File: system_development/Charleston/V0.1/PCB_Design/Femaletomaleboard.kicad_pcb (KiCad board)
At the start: 2 copper layers, 64.4 x 118.3 mm, 7 parts, among them SW2 MC74VHC1G66DFT1G

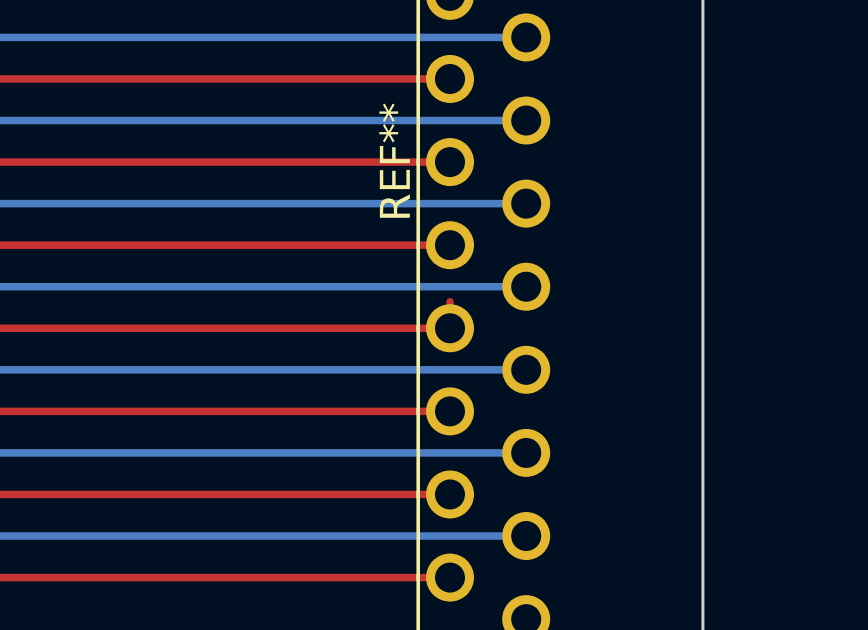
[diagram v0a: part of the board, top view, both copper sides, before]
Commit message: femaletomaleboard
Fingers crossed final version
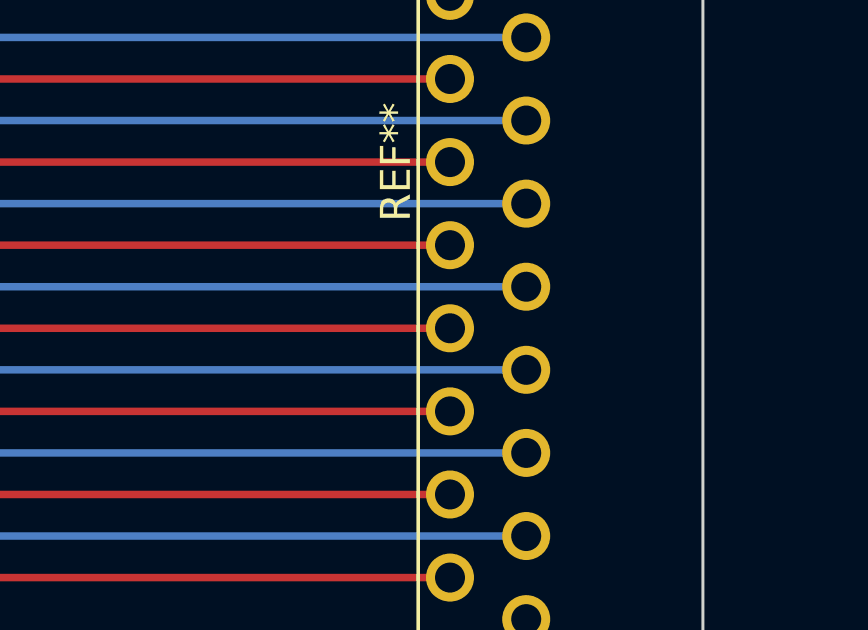
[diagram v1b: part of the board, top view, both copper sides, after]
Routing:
- net (no net): track 2812.3 -> 2811.5 mm
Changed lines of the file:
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@@
   (segment (start 142.325948 110.855) (end 142.235473 110.764525) (width 0.25) (layer "F.Cu") (net 0))
   (segment (start 144.469667 91.365) (end 144.369667 91.465) (width 0.25) (layer "F.Cu") (net 0))
-  (segment (start 167.669667 107.985) (end 167.669667 107.1) (width 0.25) (layer "F.Cu") (net 0))
   (segment (start 142.225948 116.295) (end 141.990473 116.059525) (width 0.25) (layer "F.Cu") (net 0))
   (segment (start 155.7 151.65) (end 157.4 153.35) (width 0.25) (layer "F.Cu") (net 0))
